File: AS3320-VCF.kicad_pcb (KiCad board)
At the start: 2 copper layers, 71.2 x 131.1 mm, 70 parts, among them J1 AUDIO3_INPUT, J2 AUDIO2_INPUT, J3 AUDIO1_INPUT, J4 RES_INPUT, J5 1V/OCT_INPUT, J6 CV2_INPUT, J7 --------, J8 AUDIO_OUTPUT, U1 TL082, U2 AS3320, U3 TL082

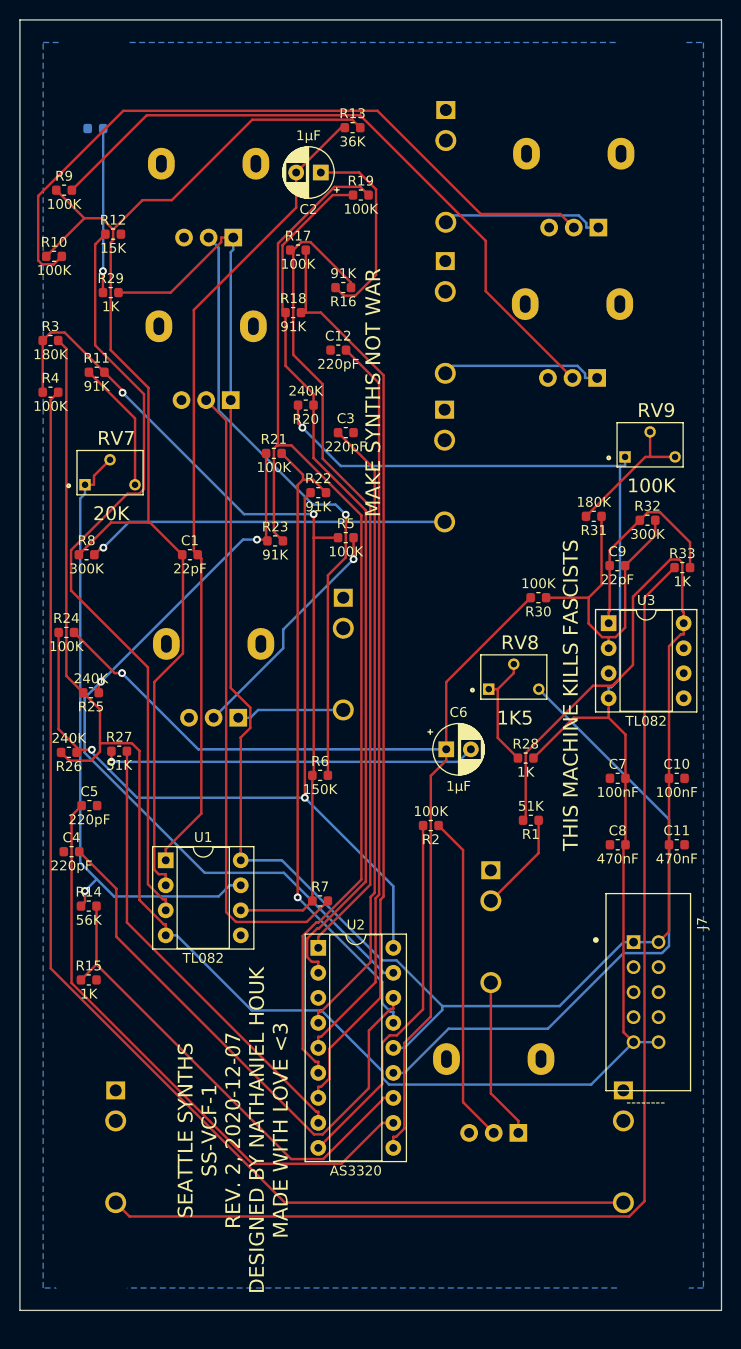
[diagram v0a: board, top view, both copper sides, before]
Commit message: Refactor board
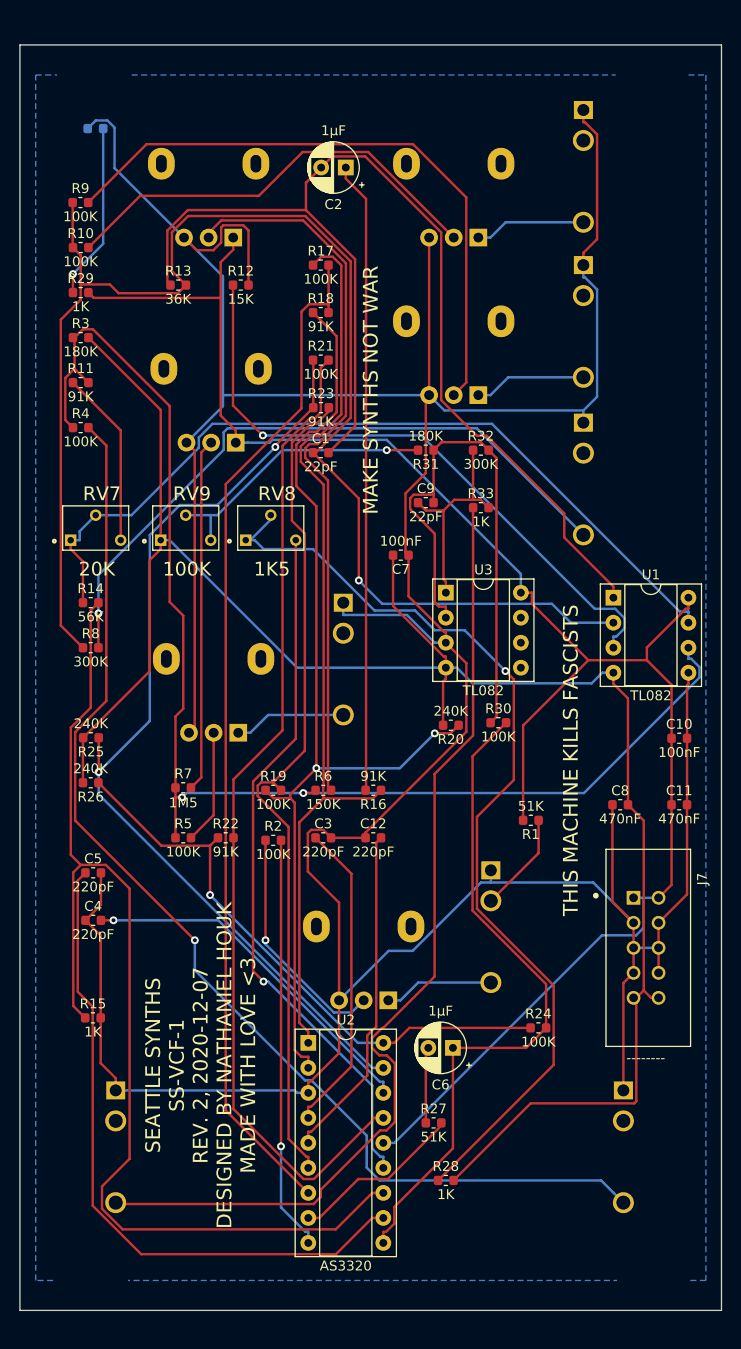
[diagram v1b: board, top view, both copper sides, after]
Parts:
- D1: value LED -> POWER
- J1: value AUDIO3_INPUT -> 3
- J2: value AUDIO2_INPUT -> 2
- J3: value AUDIO1_INPUT -> 1
- moved R24 62.5 mm to (154.4, 128.0)
- moved R19 61.1 mm to (127.5, 103.9)
- moved U1 52.7 mm to (162.1, 84.3)
- moved R16 51.1 mm to (137.7, 103.9)
- moved C12 49.7 mm to (137.7, 108.7)
- moved R27 49.4 mm to (143.8, 137.7)
- moved RV9 47.9 mm to (118.6, 78.5)
- moved R28 43.7 mm to (145.0, 143.5)
- moved C3 41.2 mm to (132.6, 108.7)
- moved R22 36.3 mm to (122.7, 108.7)
- moved R20 35.7 mm to (145.5, 97.3)
- moved R5 34.7 mm to (118.4, 108.7)
- moved C7 31.6 mm to (140.5, 80.0), turned to 180 degrees
- moved R14 30.8 mm to (109.0, 84.8)
- moved C6 30.3 mm to (145.8, 130.0), turned to 180 degrees
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- renumbered RV3 to FREQ, RV4 to RES
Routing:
- net GND: track 0.00 -> 421.0 mm
- net Net-(R28-Pad1): track 12.0 -> 97.0 mm, vias 0 -> 1
- net /VCFI: track 49.2 -> 115.2 mm
- net -12V: track 238.5 -> 192.8 mm, vias 1 -> 0
- net Net-(C2-Pad1): track 20.3 -> 64.1 mm
- net Net-(R11-Pad2): track 90.4 -> 133.3 mm
- net Net-(C12-Pad2): track 75.0 -> 34.2 mm
- net /OUT4: track 104.5 -> 68.7 mm, vias 1 -> 0
- net /OUT3: track 66.0 -> 101.2 mm, vias 1 -> 0
- net Net-(C3-Pad1): track 64.0 -> 31.9 mm
- net Net-(C1-Pad2): track 82.8 -> 114.2 mm
- net Net-(J1-PadT): track 37.0 -> 68.3 mm
- net Net-(C6-Pad2): track 38.1 -> 7.73 mm, vias 1 -> 0
- net +12V: track 212.0 -> 182.6 mm
- net Net-(R22-Pad1): track 88.4 -> 59.5 mm, vias 2 -> 1
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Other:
- board size 71.2 x 131.1 mm -> 71.2 x 128.5 mm
